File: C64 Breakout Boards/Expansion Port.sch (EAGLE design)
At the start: 2 parts, among them X1 87758-4416, X2 87758-4416

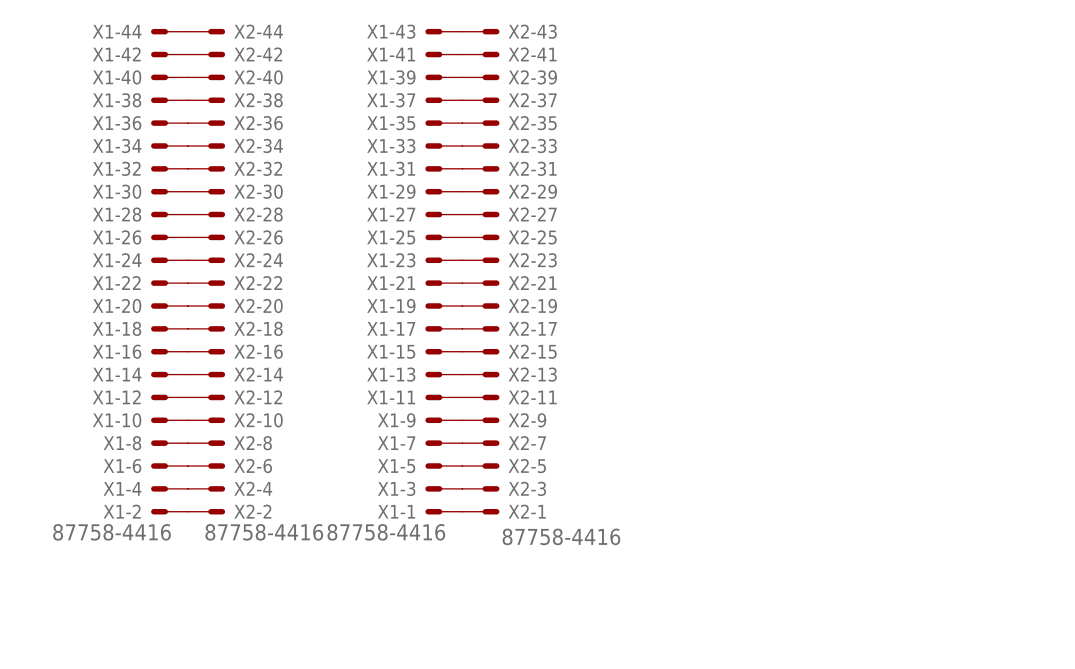
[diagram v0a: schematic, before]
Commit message: More expansion board work
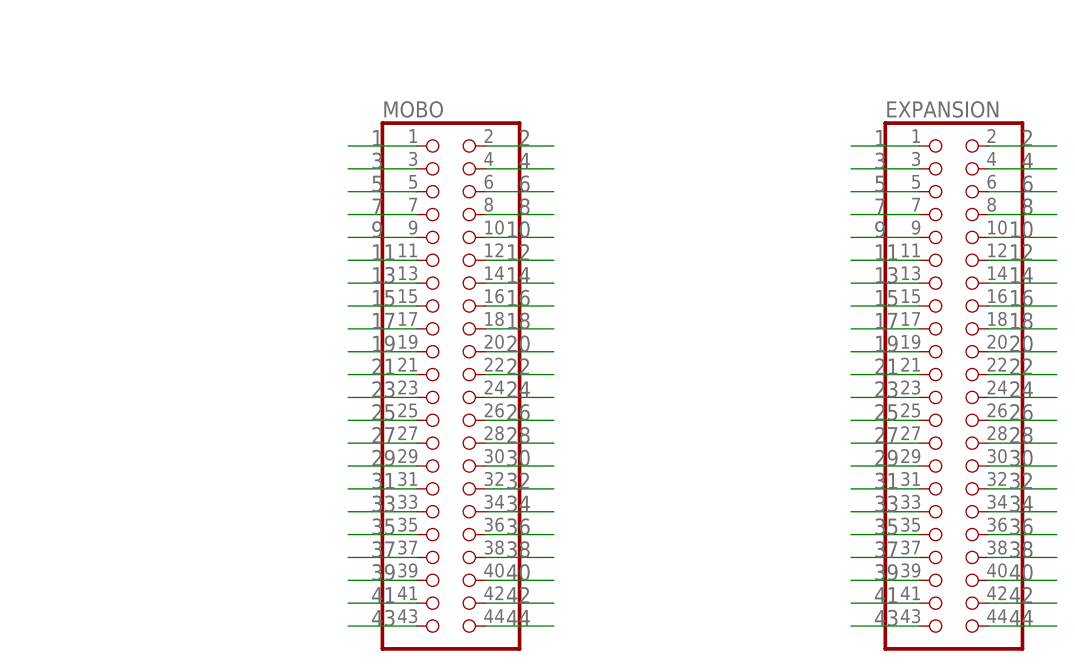
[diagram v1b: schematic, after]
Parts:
- removed X1, X2: 87758-4416, con-molex:87758-4416
- added EXPANSION, MOBO: (no value), pinhead:PINHD-2X22
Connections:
- removed net N$1: X1-1.S, X2-1.S
- removed net N$10: X1-19.S, X2-19.S
- removed net N$11: X1-21.S, X2-21.S
- removed net N$12: X1-23.S, X2-23.S
- removed net N$13: X1-25.S, X2-25.S
- removed net N$14: X1-27.S, X2-27.S
- removed net N$15: X1-29.S, X2-29.S
- removed net N$16: X1-31.S, X2-31.S
- removed net N$17: X1-33.S, X2-33.S
- removed net N$18: X1-35.S, X2-35.S
- removed net N$19: X1-37.S, X2-37.S
- removed net N$2: X1-3.S, X2-3.S
- removed net N$20: X1-39.S, X2-39.S
- removed net N$21: X1-41.S, X2-41.S
- removed net N$22: X1-43.S, X2-43.S
- removed net N$23: X1-2.S, X2-2.S
- removed net N$24: X1-4.S, X2-4.S
- removed net N$25: X1-6.S, X2-6.S
- removed net N$26: X1-8.S, X2-8.S
- removed net N$27: X1-10.S, X2-10.S
- removed net N$28: X1-12.S, X2-12.S
- removed net N$29: X1-14.S, X2-14.S
- removed net N$3: X1-5.S, X2-5.S
- removed net N$30: X1-16.S, X2-16.S
- removed net N$31: X1-18.S, X2-18.S
- removed net N$32: X1-20.S, X2-20.S
- removed net N$33: X1-22.S, X2-22.S
- removed net N$34: X1-24.S, X2-24.S
- removed net N$35: X1-26.S, X2-26.S
- removed net N$36: X1-28.S, X2-28.S
- removed net N$37: X1-30.S, X2-30.S
- removed net N$38: X1-32.S, X2-32.S
- removed net N$39: X1-34.S, X2-34.S
- removed net N$4: X1-7.S, X2-7.S
- removed net N$40: X1-36.S, X2-36.S
- removed net N$41: X1-38.S, X2-38.S
- removed net N$42: X1-40.S, X2-40.S
- removed net N$43: X1-42.S, X2-42.S
- removed net N$44: X1-44.S, X2-44.S
- removed net N$5: X1-9.S, X2-9.S
- removed net N$6: X1-11.S, X2-11.S
- removed net N$7: X1-13.S, X2-13.S
- removed net N$8: X1-15.S, X2-15.S
- removed net N$9: X1-17.S, X2-17.S
- new net 1: EXPANSION.1, MOBO.1
- new net 10: EXPANSION.10, MOBO.10
- new net 11: EXPANSION.11, MOBO.11
- new net 12: EXPANSION.12, MOBO.12
- new net 13: EXPANSION.13, MOBO.13
- new net 14: EXPANSION.14, MOBO.14
- new net 15: EXPANSION.15, MOBO.15
- new net 16: EXPANSION.16, MOBO.16
- new net 17: EXPANSION.17, MOBO.17
- new net 18: EXPANSION.18, MOBO.18
- new net 19: EXPANSION.19, MOBO.19
- new net 2: EXPANSION.2, MOBO.2
- new net 20: EXPANSION.20, MOBO.20
- new net 21: EXPANSION.21, MOBO.21
- new net 22: EXPANSION.22, MOBO.22
- new net 23: EXPANSION.23, MOBO.23
- new net 24: EXPANSION.24, MOBO.24
- new net 25: EXPANSION.25, MOBO.25
- new net 26: EXPANSION.26, MOBO.26
- new net 27: EXPANSION.27, MOBO.27
- new net 28: EXPANSION.28, MOBO.28
- new net 29: EXPANSION.29, MOBO.29
- new net 3: EXPANSION.3, MOBO.3
- new net 30: EXPANSION.30, MOBO.30
- new net 31: EXPANSION.31, MOBO.31
- new net 32: EXPANSION.32, MOBO.32
- new net 33: EXPANSION.33, MOBO.33
- new net 34: EXPANSION.34, MOBO.34
- new net 35: EXPANSION.35, MOBO.35
- new net 36: EXPANSION.36, MOBO.36
- new net 37: EXPANSION.37, MOBO.37
- new net 38: EXPANSION.38, MOBO.38
- new net 39: EXPANSION.39, MOBO.39
- new net 4: EXPANSION.4, MOBO.4
- new net 40: EXPANSION.40, MOBO.40
- new net 41: EXPANSION.41, MOBO.41
- new net 42: EXPANSION.42, MOBO.42
- new net 43: EXPANSION.43, MOBO.43
- new net 44: EXPANSION.44, MOBO.44
- new net 5: EXPANSION.5, MOBO.5
- new net 6: EXPANSION.6, MOBO.6
- new net 7: EXPANSION.7, MOBO.7
- new net 8: EXPANSION.8, MOBO.8
- new net 9: EXPANSION.9, MOBO.9
